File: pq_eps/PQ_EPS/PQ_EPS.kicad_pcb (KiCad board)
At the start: 4 copper layers, 40 x 40 mm, 89 parts, among them IC1 DS2782E+, IC2 ISL9120IRTNZ, J1 CES-110-02-L-S, J2 CES-110-02-L-S, J3 CES-110-02-L-S, J4 CES-110-02-L-S, Q1 SIR424DP, U1 SPV1040TTR, U2 SPV1040TTR, U3 SPV1040TTR, U4 LTC4040EUFD#PBF

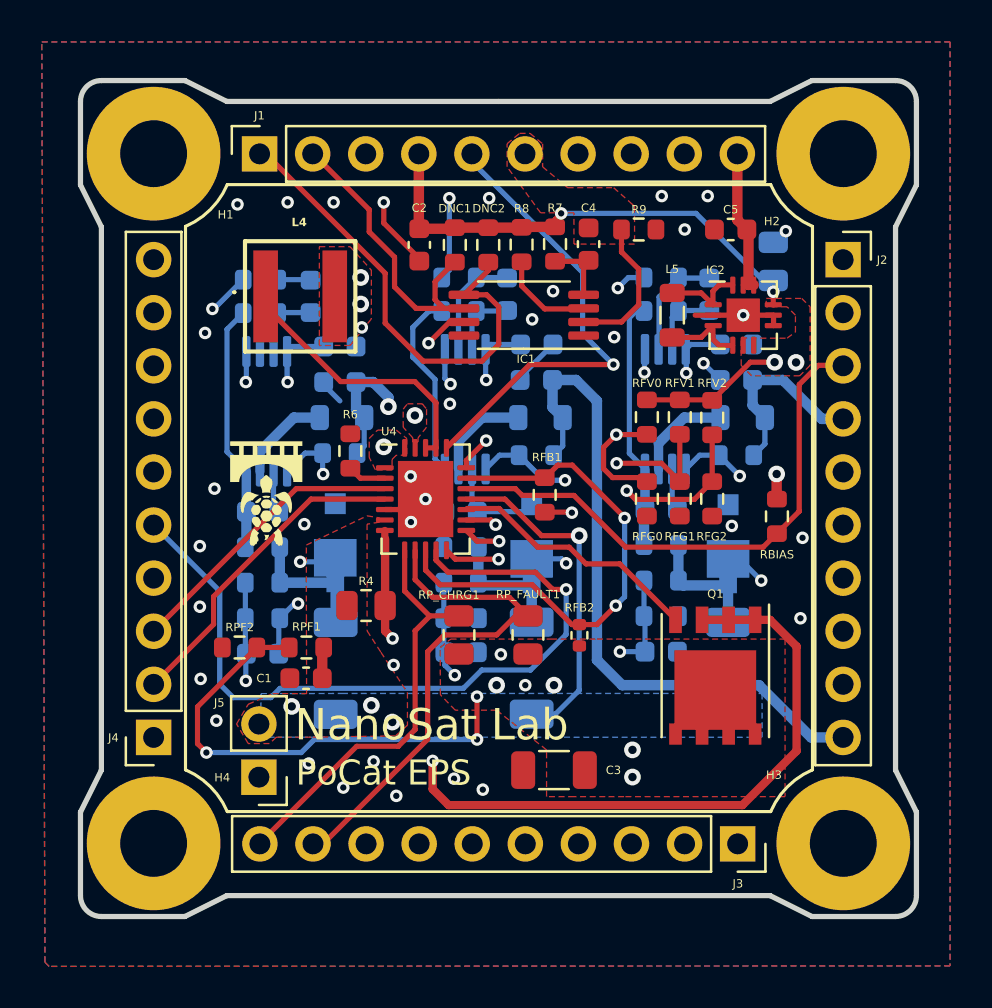
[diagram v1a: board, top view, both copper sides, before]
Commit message: EPS corrected and verified. Production ready
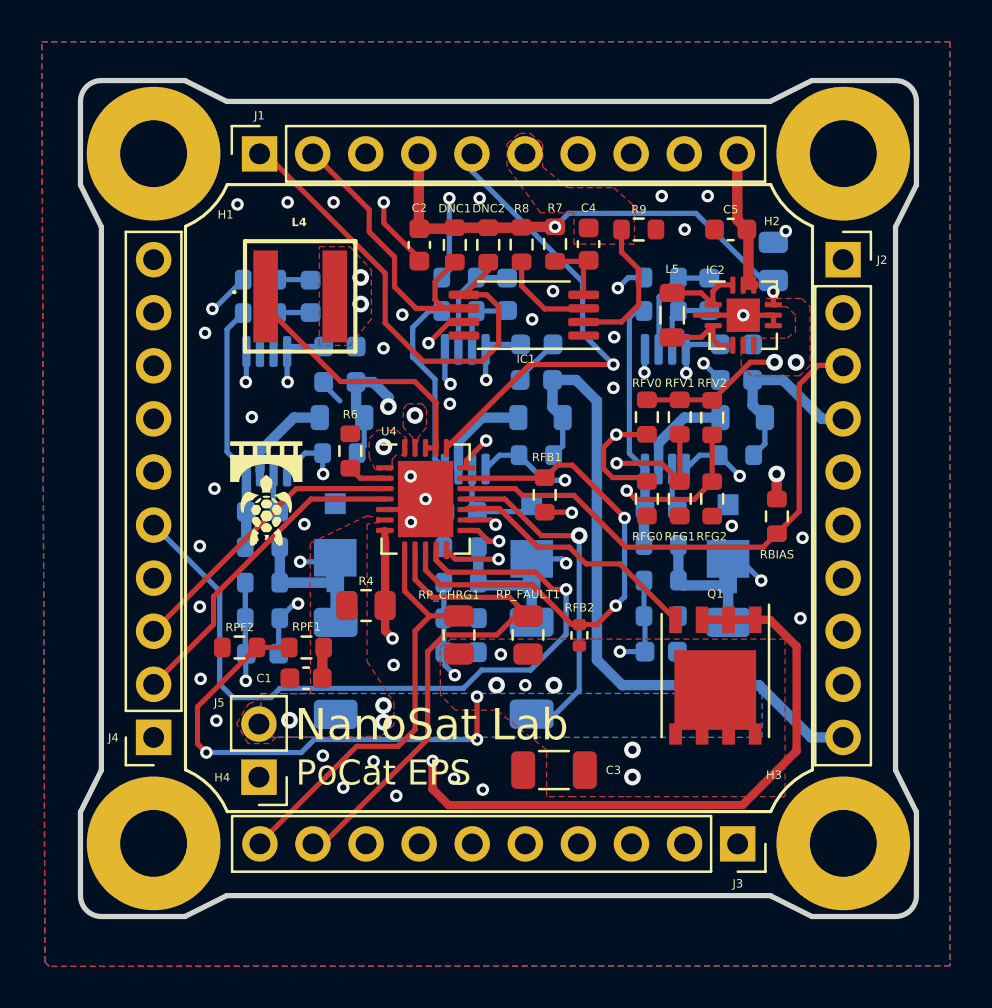
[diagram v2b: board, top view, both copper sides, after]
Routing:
- net GND: vias 41 -> 44
